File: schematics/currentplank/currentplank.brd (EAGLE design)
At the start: 80 x 49 mm, 24 parts, among them IC1 74AHC1G86DBV, IC2 STCS2A, IC3 STCS2A

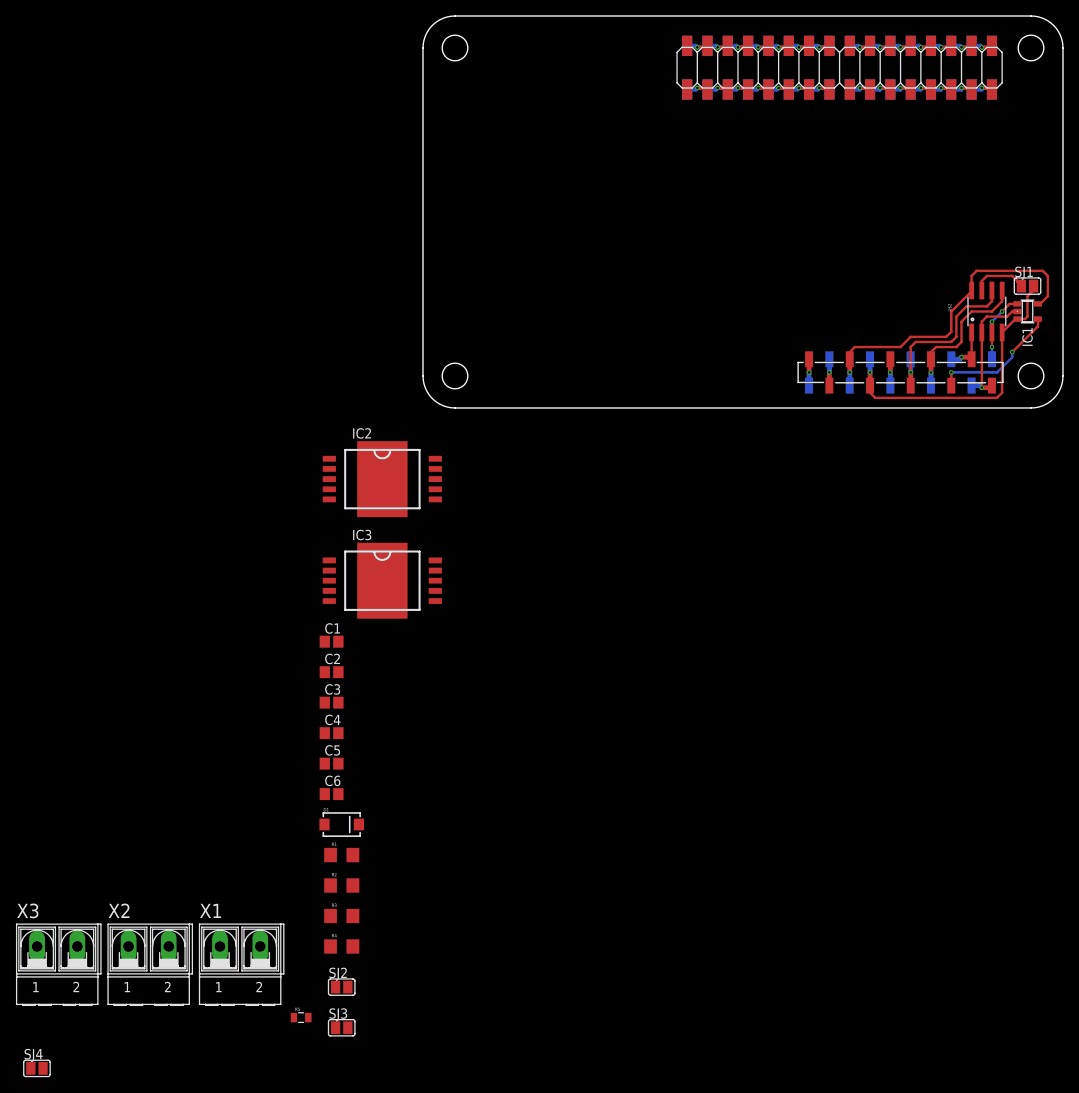
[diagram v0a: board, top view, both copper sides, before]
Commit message: Work on constant current plank.
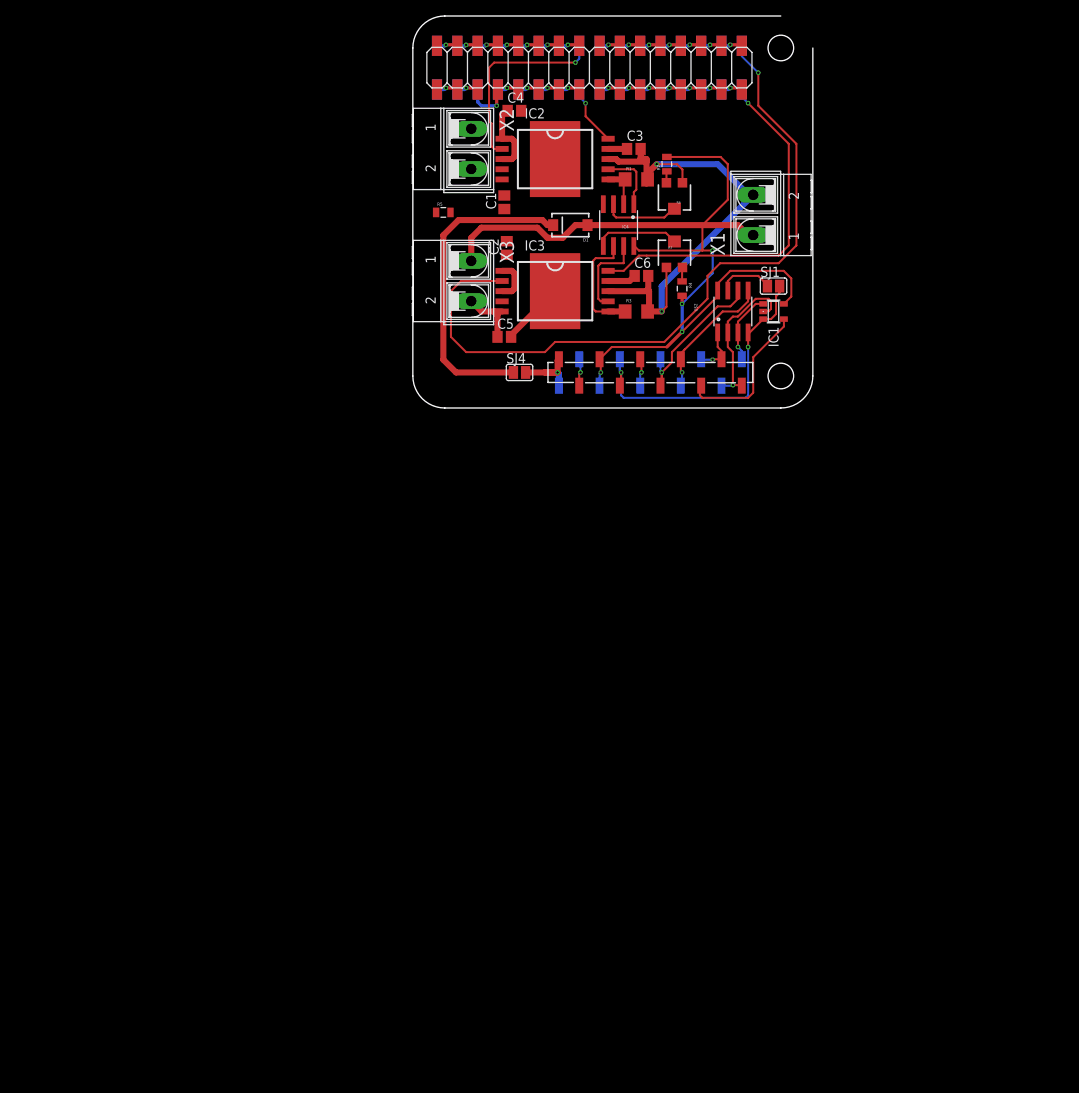
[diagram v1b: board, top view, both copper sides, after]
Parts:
- removed SJ2, SJ3: (no value), jumper:SJ
- added IC4: OPAMP-DUALU, SparkFun-AnalogIC:SO08
- added R6, R7: 1k, nickparts:TRIMPOT-3MM-2
- R1, R3: value .1 ohm -> 0.05
- R2, R4: value .1 ohm -> 32k; device SparkFun-Passives:1206 -> SparkFun-Passives:0805
- U$1: value LOKI_PLANKLONG -> LOKI_PLANKSHORT; device loki:PLANK_LONG -> loki:PLANK_SHORT
- moved X1 111.7 mm to (42.5, 24.1), turned to 90 degrees
- moved X2 107.5 mm to (7.30, 32.4), turned to 270 degrees
- moved SJ4 105.9 mm to (13.3, 4.45)
- moved R5 102.2 mm to (3.81, 24.4)
- moved R2 98.9 mm to (31.8, 30.5), turned to 90 degrees
- moved X3 98.0 mm to (7.30, 15.9), turned to 270 degrees
- moved R4 92.6 mm to (33.7, 14.9), turned to 270 degrees
- moved R1 92.1 mm to (27.9, 28.6)
- moved R3 84.1 mm to (27.9, 12.1)
- moved C4 81.1 mm to (12.7, 37.1)
- moved D1 80.2 mm to (19.7, 22.9), turned to 180 degrees
- moved C3 78.9 mm to (27.6, 32.4)
- moved C6 75.5 mm to (28.6, 16.5)
- moved C1 59.0 mm to (11.4, 25.7), turned to 90 degrees
- moved C5 57.5 mm to (11.4, 8.89)
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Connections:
- new net DISC2: IC3.10, U$1.I1.2
- new net N$43: R2.1, R6.3
- new net N$44: IC4.5, R7.2
- new net N$45: R4.1, R7.3
- new net N$46: C2.1, C4.1, IC2.1, IC2.3, IC3.1, IC3.3, R5.1
- new net PWM2: IC3.2, U$1.I1.1
- net +3V3: now also IC4.8, R2.2, R4.2
- net DISC1: now also U$1.I2.2; no longer U$1.I1.2
- net GND: now also IC4.4, R6.1, R7.1; no longer R2.2, R4.2
- net N$29: now also IC4.2; no longer IC2.7, SJ2.1
- net N$30: now also IC2.7, IC4.1; no longer R2.1, SJ2.2
- net N$33: now also D1.C, R5.2, SJ4.1; no longer D1.A, X1.1
- net N$35: now also D1.A, X1.1, X2.1, X3.1; no longer D1.C, R5.1, SJ4.1
- net N$36: now also IC4.3, R6.2; no longer C2.1, C4.1, IC2.1, IC2.3, IC3.1, IC3.3, R5.2, X2.2, X3.2
- net N$37: now also X2.2; no longer X2.1
- net N$38: now also X3.2; no longer X3.1
- net N$41: now also IC3.6, IC4.6; no longer IC3.7, SJ3.1
- net N$42: now also IC3.7, IC4.7; no longer R4.1, SJ3.2
- net PWM1: now also U$1.I2.1; no longer U$1.I1.1
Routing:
- net PWM2: track 0.00 -> 91.6 mm, vias 0 -> 1
- net GND: track 36.9 -> 117.6 mm, vias 1 -> 4
- net DISC2: track 0.00 -> 45.8 mm, vias 0 -> 1
- net +3V3: track 40.2 -> 83.4 mm, vias 1 -> 4
- net N$35: track 0.00 -> 40.4 mm
- net N$33: track 0.00 -> 39.8 mm
- net PWM1: track 0.00 -> 24.8 mm, vias 0 -> 1
- net N$41: track 0.00 -> 14.3 mm
- net N$46: track 0.00 -> 13.6 mm
- net N$42: track 0.00 -> 10.9 mm
- net N$44: track 0.00 -> 10.6 mm
- net N$36: track 0.00 -> 9.55 mm
- net N$30: track 0.00 -> 7.85 mm
- net N$38: track 0.00 -> 7.74 mm
- net DISC1: track 0.00 -> 7.65 mm, vias 0 -> 1
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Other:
- board size 80 x 49 mm -> 50 x 49 mm
